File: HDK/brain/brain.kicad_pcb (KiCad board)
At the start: 2 copper layers, 48 x 48 mm, 29 parts, among them J301 Can Conn, J303 Can Conn, J305 Can Conn, J307 Can Conn, U201 W25Q128JVS, U202 RP2040, U401 ADS1015IDGS, U402 ASSR-1218, U501 LR7533-T LR, Y201 12 MHz

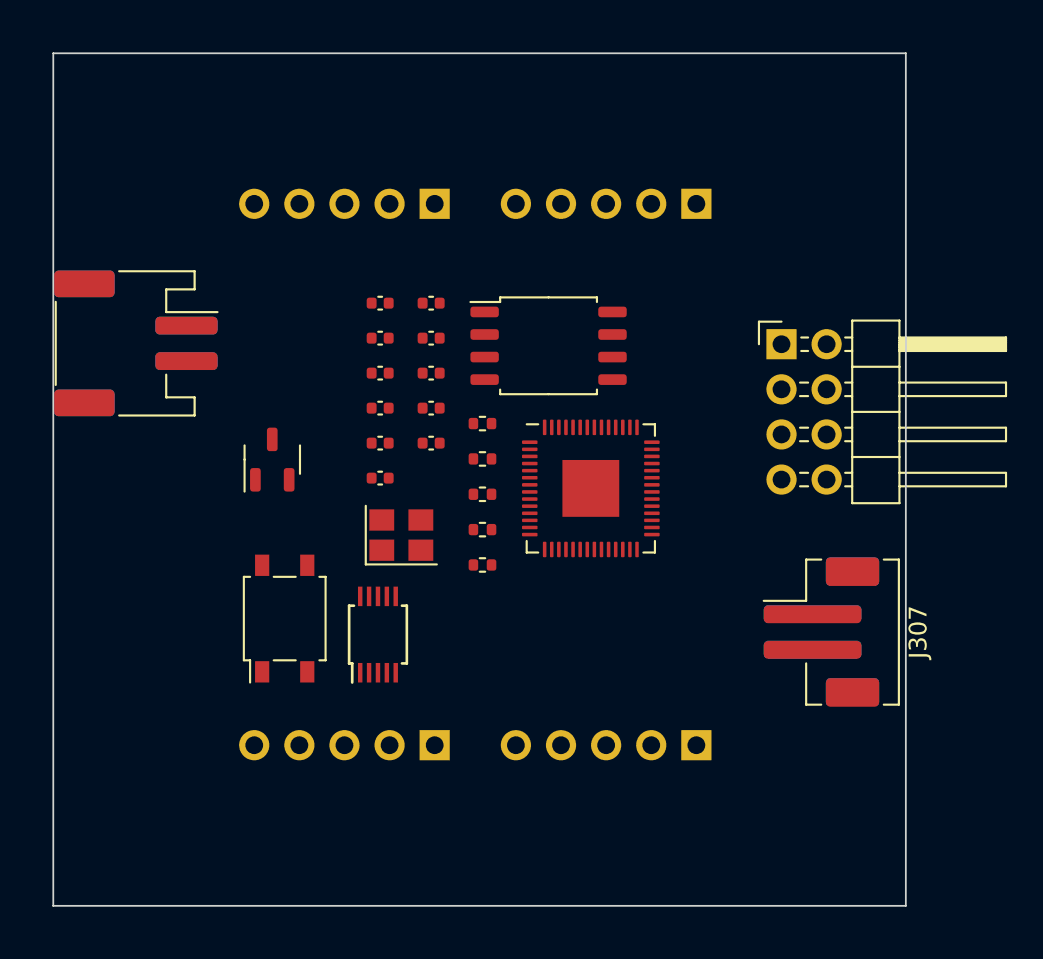
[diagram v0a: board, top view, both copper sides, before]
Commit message: updated brain
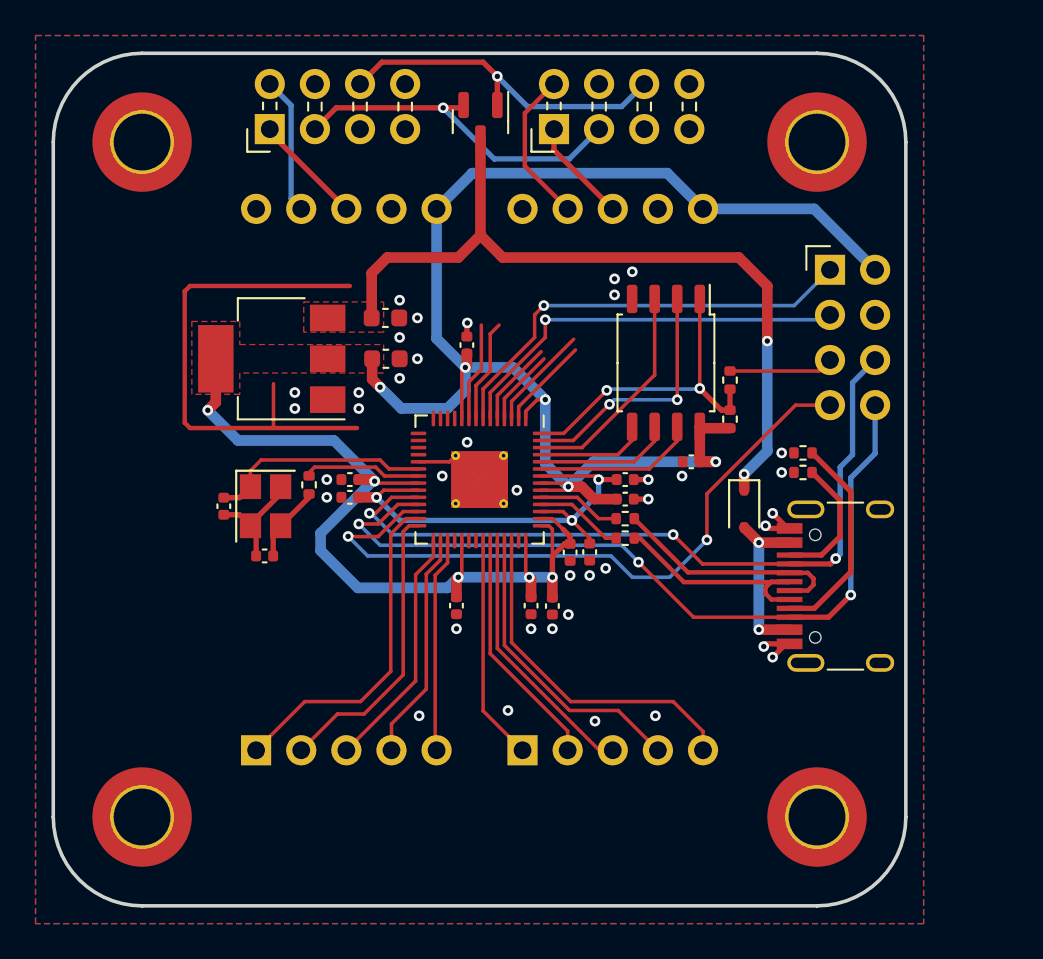
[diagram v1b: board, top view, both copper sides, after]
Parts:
- removed the J305 at (143.2, 132.6)
- removed J307: Can Conn, Connector_JST:JST_PH_B2B-PH-SM4-TB_1x02-1MP_P2.00mm_Vertical
- removed the REF** at (141.0, 116.4)
- removed U402: ASSR-1218, Package_SO:SO-4_4.4x4.3mm_P2.54mm
- removed U501: LR7533-T LR, Package_TO_SOT_SMD:SOT-23-3
- added C212: 10p, Capacitor_SMD:C_0402_1005Metric, F.Cu at (109.6, 125.5)
- added C213: 10p, Capacitor_SMD:C_0402_1005Metric, F.Cu at (111.9, 128.3)
- added C401: 4.7u, Capacitor_SMD:C_0603_1608Metric, F.Cu at (118.7, 114.9)
- added C402: 4.7u, Capacitor_SMD:C_0603_1608Metric, F.Cu at (118.7, 117.2)
- added D401: BAV70, Package_TO_SOT_SMD:SOT-23, F.Cu at (124.0, 103.8)
- added D402: 1N5819WS, Diode_SMD:D_SOD-323, F.Cu at (138.9, 125.7)
- added J302: uC Interconnect, NVF-Kicad:2x04H-S, F.Cu at (132.0, 103.0)
- added J306: USB_C, Connector_USB:USB_C_Receptacle_HRO_TYPE-C-31-M-12, F.Cu at (145.5, 130.0)
- added R301: 5k1, Resistor_SMD:R_0402_1005Metric, F.Cu at (142.2, 122.5)
- added R302: 5k1, Resistor_SMD:R_0402_1005Metric, F.Cu at (142.2, 123.6)
- added REF**: MountingHole_3.2mm_M3_DIN965_Pad_TopOnly, MountingHole:MountingHole_3.2mm_M3_DIN965_Pad_TopOnly, F.Cu at (105.0, 143.0)
- added REF**: MountingHole_3.2mm_M3_DIN965_Pad_TopOnly, MountingHole:MountingHole_3.2mm_M3_DIN965_Pad_TopOnly, F.Cu at (105.0, 105.0)
- added REF**: MountingHole_3.2mm_M3_DIN965_Pad_TopOnly, MountingHole:MountingHole_3.2mm_M3_DIN965_Pad_TopOnly, F.Cu at (143.0, 143.0)
- added REF**: MountingHole_3.2mm_M3_DIN965_Pad_TopOnly, MountingHole:MountingHole_3.2mm_M3_DIN965_Pad_TopOnly, F.Cu at (143.0, 105.0)
- C207: renamed from C206; value 100n -> 1u
- C209: renamed from C210; value 10p -> 100n
- C210: renamed from C209; value 100n -> 1u
- C211: value 10p -> 100n
- J301: value Can Conn -> uC Interconnect; footprint Connector_JST:JST_PH_S2B-PH-SM4-TB_1x02-1MP_P2.00mm_Horizontal -> NVF-Kicad:2x04H-S; moved to F.Cu
- J303: value Can Conn -> DBG Connect; footprint Connector_JST:JST_PH_S2B-PH-SM4-TB_1x02-1MP_P2.00mm_Horizontal -> NVF-Kicad:2x04V-S
- J304, J305: renamed from REF**; value Can Module 2515 -> MCP251X; footprint NVF-Kicad:Can Module 2515 -> NVF-Kicad:Can-Module-CM251X
- U202: footprint Package_DFN_QFN:QFN-56-1EP_7x7mm_P0.4mm_EP3.2x3.2mm -> Package_DFN_QFN:QFN-56-1EP_7x7mm_P0.4mm_EP3.2x3.2mm_ThermalVias
- U401: value ADS1015IDGS -> AMS1117-3.3; footprint Package_SO:TSSOP-10_3x3mm_P0.5mm -> Package_TO_SOT_SMD:SOT-223-3_TabPin2
- moved J303 40.4 mm to (145.0, 116.0)
- moved C206 18.4 mm to (128.1, 131.1), turned to -90 degrees
- moved C201 17.7 mm to (132.2, 125.1)
- moved J301 17.5 mm to (116.0, 103.0), turned to 0 degrees
- moved U401 16.6 mm to (112.3, 117.2), turned to 180 degrees
- moved R204 15.3 mm to (138.1, 120.6), turned to 90 degrees
- moved C211 14.7 mm to (135.9, 123.0), turned to 180 degrees
- moved R201 14.1 mm to (138.1, 118.4), turned to 90 degrees
- moved C210 13.5 mm to (130.2, 128.1), turned to -90 degrees
- moved C205 12.5 mm to (126.9, 131.1), turned to -90 degrees
- moved C204 11.9 mm to (122.7, 131.1), turned to -90 degrees
- moved C209 11.6 mm to (132.2, 124.0)
- moved C207 11.5 mm to (129.1, 128.1), turned to -90 degrees
- moved R205 10.8 mm to (114.4, 124.3), turned to 90 degrees
- moved C208 10.1 mm to (116.7, 125.0), turned to 180 degrees
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- renumbered C207 to C206
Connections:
- net Net-(U202-USB_DM) renamed /Controller/USB_DtN
- net Net-(U202-USB_DP) renamed /Controller/USB_DtP
- C209 pad 1: /Controller/HSE_IN -> +1V1
- C211 pad 1: /Controller/HSE_OUT -> +3V3
- J301 pad 1: /Connectors/CAN1_L -> /Connectors/CAN1_H
- J301 pad 2: /Connectors/CAN1_H -> /Connectors/CAN1_L
- J303 pad 1: /Connectors/CAN1_L -> /Connectors/UART1_RX
- J303 pad 2: /Connectors/CAN1_H -> +3V3
- J304 pad 1: (no net) -> /SPI0_CS1
- J304 pad 10: (no net) -> +3V3
- J304 pad 2: (no net) -> /CAN2_INT
- J304 pad 3: (no net) -> /Connectors/SPI0_SCLK
- J304 pad 4: (no net) -> /Connectors/SPI0_MOSI
- J304 pad 5: (no net) -> /Connectors/SPI0_MISO
- J304 pad 6: (no net) -> /Connectors/SOF1
- J304 pad 7: (no net) -> /Connectors/CAN1_L
- J304 pad 8: (no net) -> /Connectors/CAN1_H
- J304 pad 9: (no net) -> GND
- J305 pad 1: (no net) -> /SPI1_CS1
- J305 pad 10: (no net) -> +3V3
- J305 pad 2: (no net) -> /CAN1_INT
- J305 pad 3: (no net) -> /Connectors/SPI1_SCLK
- J305 pad 4: (no net) -> /Connectors/SPI1_MOSI
- J305 pad 5: (no net) -> /Connectors/SPI1_MISO
- J305 pad 6: (no net) -> /Connectors/SOF2
- J305 pad 7: (no net) -> /Connectors/CAN2_L
- J305 pad 8: (no net) -> /Connectors/CAN2_H
- J305 pad 9: (no net) -> GND
- R201 pad 2: /Controller/BOOT -> /Connectors/BOOT
- R203 pad 1: /Connectors/USB_DM -> /Connectors/USB_DN
- U202 pad 11: /I2C0_SDA -> /Controller/GP8
- U202 pad 12: /I2C0_SCL -> /Controller/GP9
- U202 pad 13: /Connectors/SPI1_SCLK -> /Controller/GP10
- U202 pad 14: /Connectors/SPI1_MOSI -> /Controller/GP11
- U202 pad 15: /Connectors/SPI1_MISO -> /Controller/GP12
- U202 pad 26: /Controller/~{NRST} -> /Connectors/~{NRST}
- U202 pad 27: /Controller/GP16 -> /SPI0_CS1
- U202 pad 28: /Controller/GP17 -> /CAN2_INT
- U202 pad 36: /Controller/GP24 -> /SPI1_CS1
- U202 pad 37: /Controller/GP25 -> /CAN1_INT
- U202 pad 38: /Controller/GP26 -> /Connectors/SPI1_SCLK
- U202 pad 39: /Controller/GP27 -> /Connectors/SPI1_MOSI
- U202 pad 40: /Controller/GP28 -> /Connectors/SPI1_MISO
- U202 pad 6: /Controller/GP4 -> /Connectors/UART1_TX
- U202 pad 7: /Controller/GP5 -> /Connectors/UART1_RX
- U401 pad 2: /Peripherals/ADC_IRQ -> +3V3
- U401 pad 3: GND -> /Power/V_{IN}
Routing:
- net +3V3: track 0.00 -> 135.6 mm, vias 0 -> 10
- net /Connectors/SWDIO: track 0.00 -> 45.5 mm, vias 0 -> 3
- net /Power/V_{IN}: track 0.00 -> 44.4 mm, vias 0 -> 2
- net /Connectors/SWCLK: track 0.00 -> 42.8 mm, vias 0 -> 3
- net /Connectors/~{NRST}: track 0.00 -> 38.2 mm, vias 0 -> 2
- net (no net): track 0.00 -> 26.6 mm
- net +1V1: track 0.00 -> 26.1 mm, vias 0 -> 3
- net /Connectors/UART1_RX: track 0.00 -> 24.7 mm, vias 0 -> 1
- net /Connectors/UART1_TX: track 0.00 -> 23.0 mm, vias 0 -> 1
- net /Connectors/V_{IN2}: track 0.00 -> 19.7 mm, vias 0 -> 1
- net /Connectors/SPI1_MISO: track 0.00 -> 19.6 mm
- net /Connectors/V_{IN1}: track 0.00 -> 19.6 mm, vias 0 -> 1
- net /SPI0_CS1: track 0.00 -> 19.1 mm
- net /Controller/QSPI_SS: track 0.00 -> 18.4 mm, vias 0 -> 2
- net /Connectors/SPI1_MOSI: track 0.00 -> 17.0 mm
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- added copper zone on F.Cu, net +3V3
- added copper zone on F.Cu, net /Power/V_{IN}
- added copper zone on B.Cu, net GND
- added copper zone on F.Cu, net GND
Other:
- outline, holes or cut-outs redrawn
